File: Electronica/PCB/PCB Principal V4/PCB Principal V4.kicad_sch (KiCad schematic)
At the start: 12 parts, among them J1 Conexion Sensores, J2 Power Monster, J3 On/Off General, J4 Power Input 2, J5 IDC Placa Botones, J6 Power Input 1, SW1 On/Off Motores

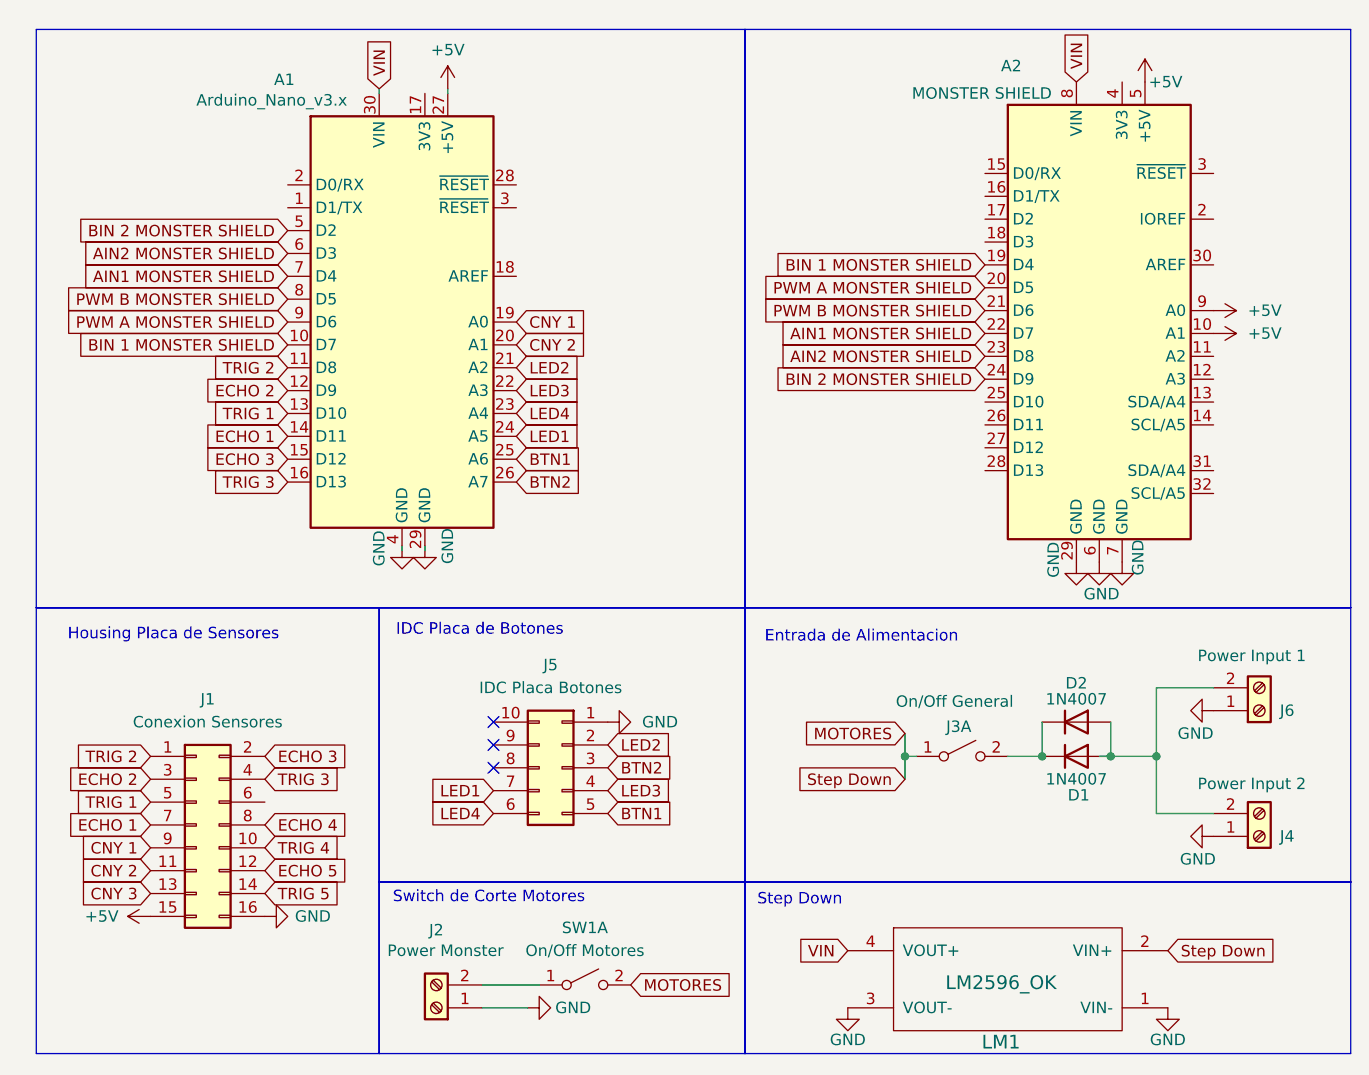
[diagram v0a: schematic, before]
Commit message: Listo PCB Botones
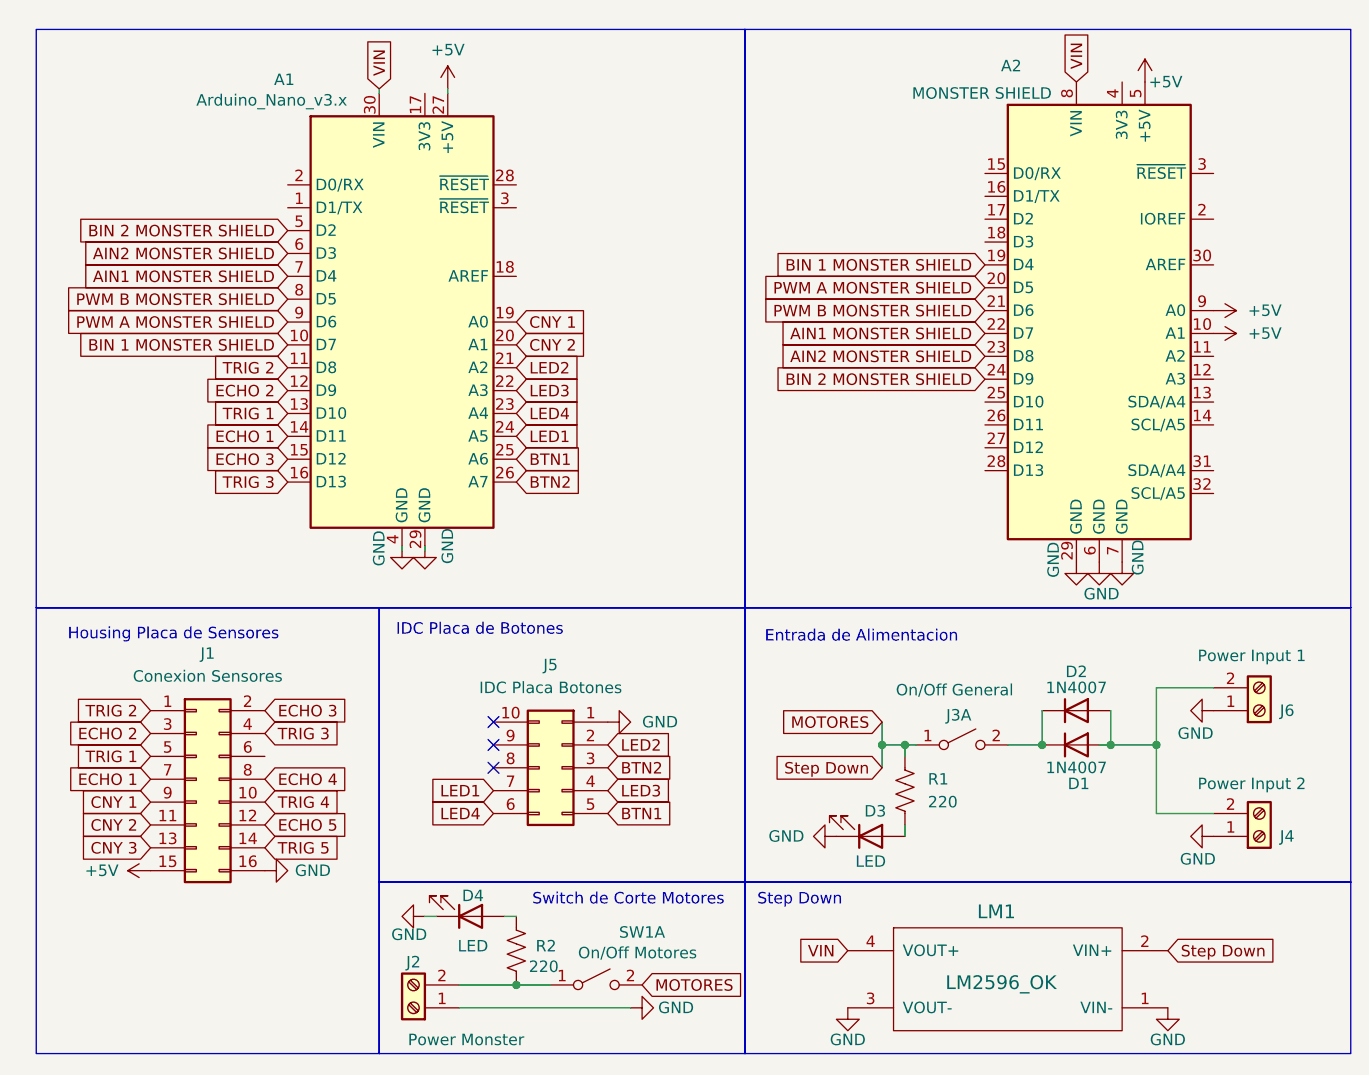
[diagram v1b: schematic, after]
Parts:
- added D3, D4: LED, LED_THT:LED_D5.0mm_Horizontal_O1.27mm_Z3.0mm, symbol Device:LED
- added R1, R2: 220, Resistor_THT:R_Axial_DIN0204_L3.6mm_D1.6mm_P5.08mm_Horizontal, symbol Device:R_US
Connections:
- net GND: now also D3.1 (K), D4.1 (K)
- net MOTORES: now also R1.1
- net at J2.2 (Pin_2), SW1.1 (A): now also R2.1
- new net: D4.2 (A), R2.2
- new net: D3.2 (A), R1.2
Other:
- moved on the sheet: D1, D2, J1, J2, J3A, SW1A

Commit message: PCB Principal con leds
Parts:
- R1, R2: footprint Resistor_THT:R_Axial_DIN0204_L3.6mm_D1.6mm_P5.08mm_Horizontal -> Resistor_THT:R_Axial_DIN0204_L3.6mm_D1.6mm_P7.62mm_Horizontal
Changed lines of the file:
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@@
 			)
 		)
-		(property "Footprint" "Resistor_THT:R_Axial_DIN0204_L3.6mm_D1.6mm_P5.08mm_Horizontal"
+		(property "Footprint" "Resistor_THT:R_Axial_DIN0204_L3.6mm_D1.6mm_P7.62mm_Horizontal"
 			(at 65.024 116.586 90)
 			(effects
@@
 			)
 		)
-		(property "Footprint" "Resistor_THT:R_Axial_DIN0204_L3.6mm_D1.6mm_P5.08mm_Horizontal"
+		(property "Footprint" "Resistor_THT:R_Axial_DIN0204_L3.6mm_D1.6mm_P7.62mm_Horizontal"
 			(at 110.236 99.314 90)
 			(effects

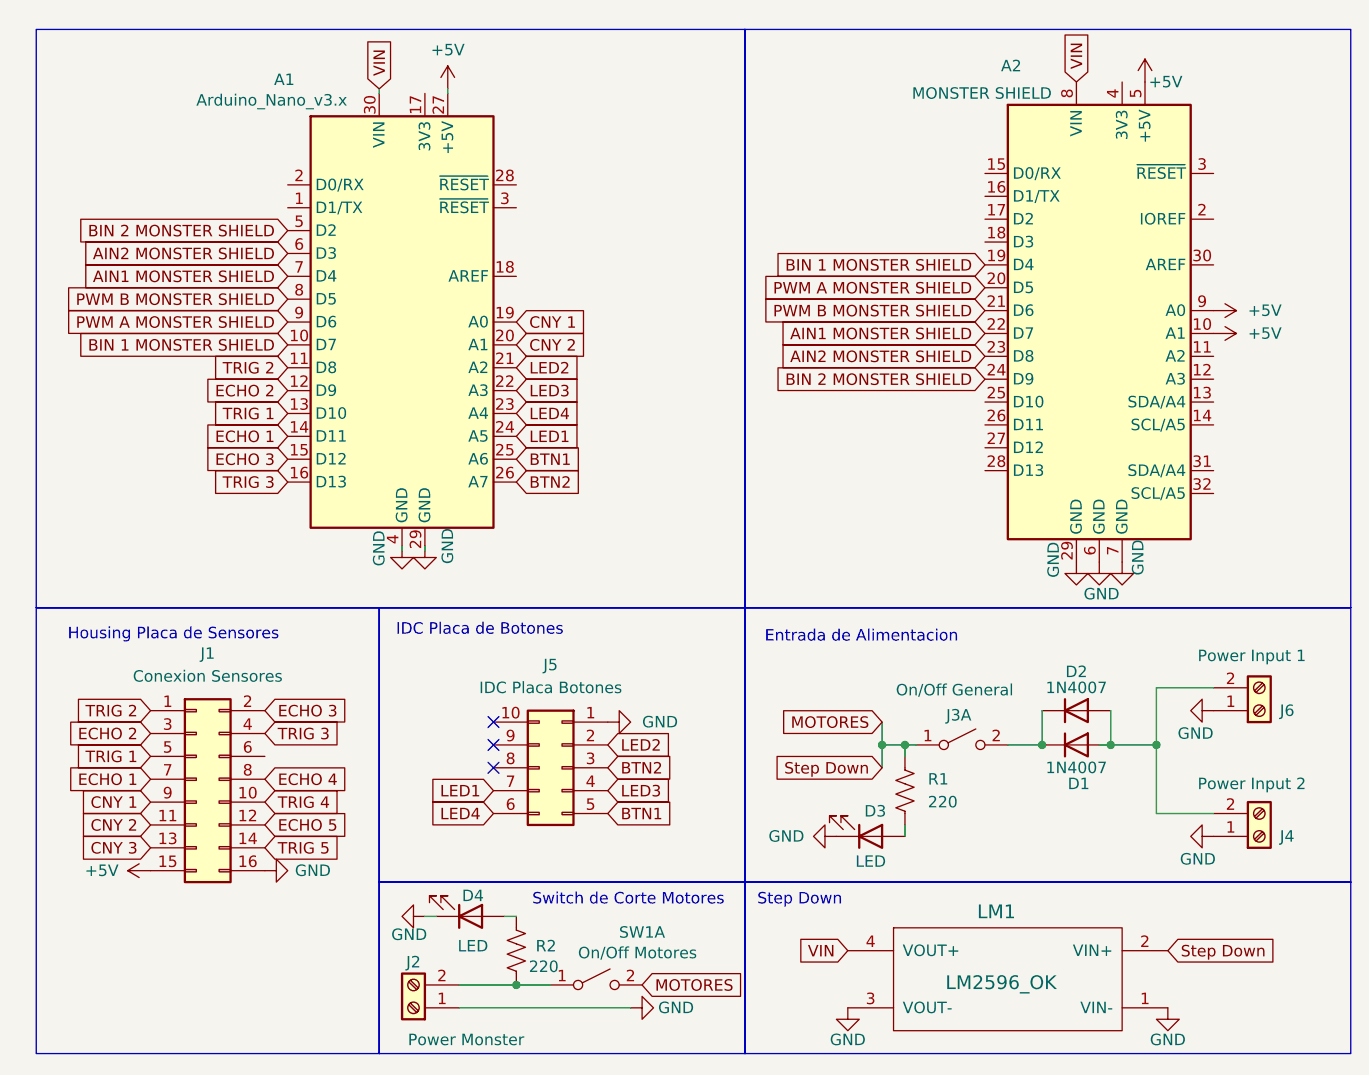
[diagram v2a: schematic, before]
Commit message: TEST POINTSSSS
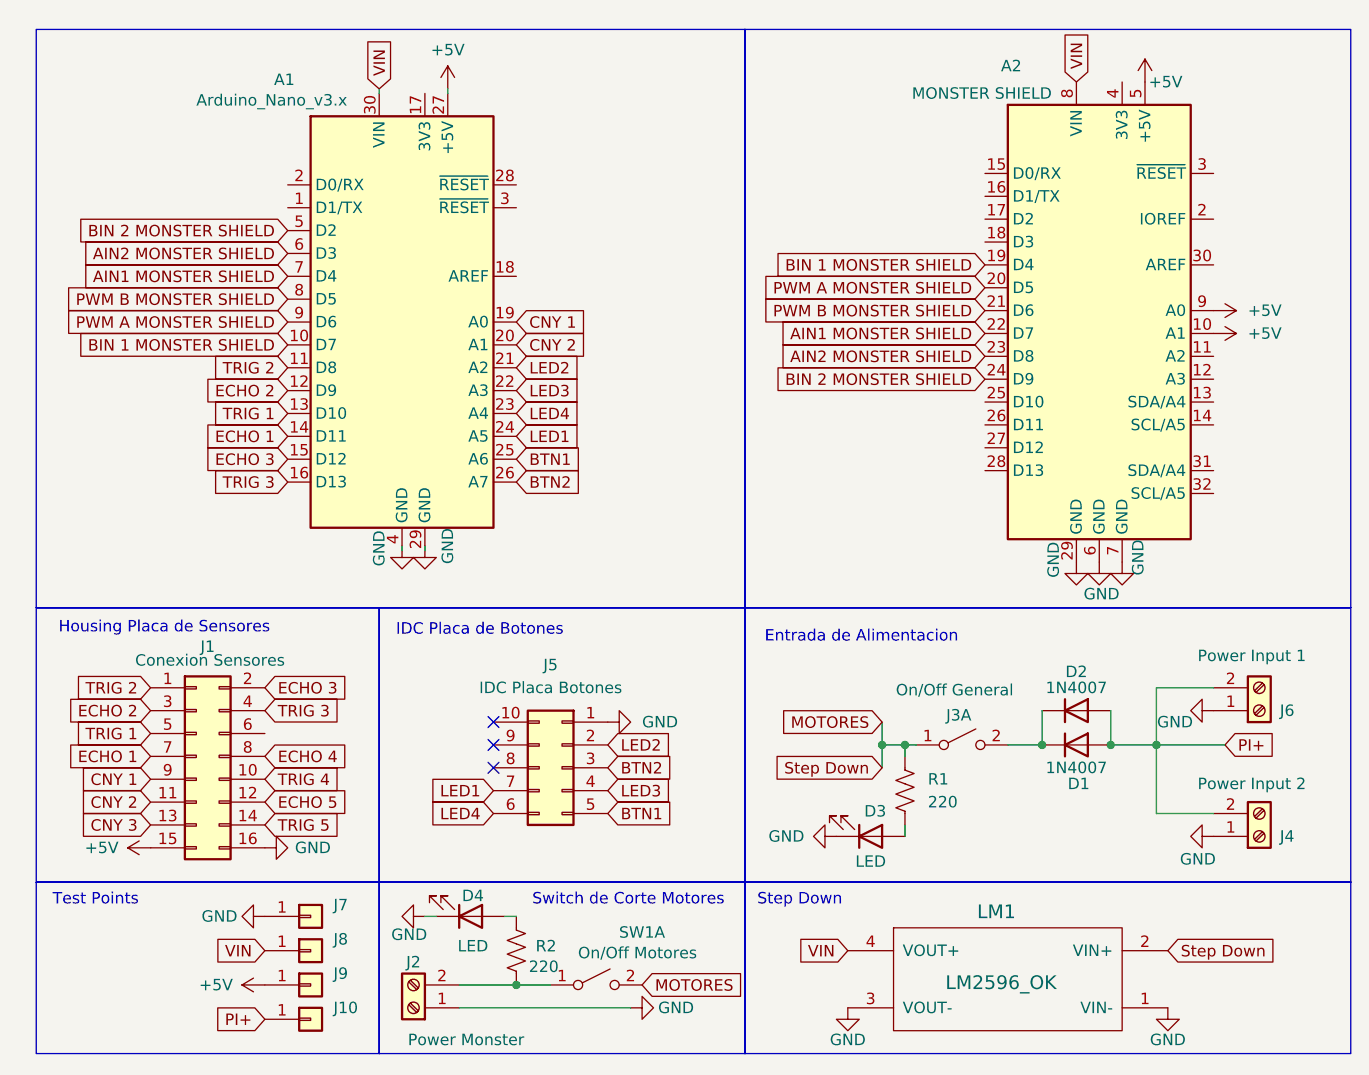
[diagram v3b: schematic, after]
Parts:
- added J10, J7, J8, J9: Conn_01x01, Connector_PinHeader_1.00mm:PinHeader_1x01_P1.00mm_Vertical, symbol Connector_Generic:Conn_01x01
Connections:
- net +5V: now also J9.1 (Pin_1)
- net GND: now also J7.1 (Pin_1)
- net VIN: now also J8.1 (Pin_1)
- net PI+: now reaches D1.2 (A), D2.2 (A), J4.2 (Pin_2), J6.2 (Pin_2)
- net PI+: now also J10.1 (Pin_1)
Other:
- note added: "Test Points"
- moved on the sheet: J1
